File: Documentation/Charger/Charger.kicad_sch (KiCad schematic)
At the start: 14 parts

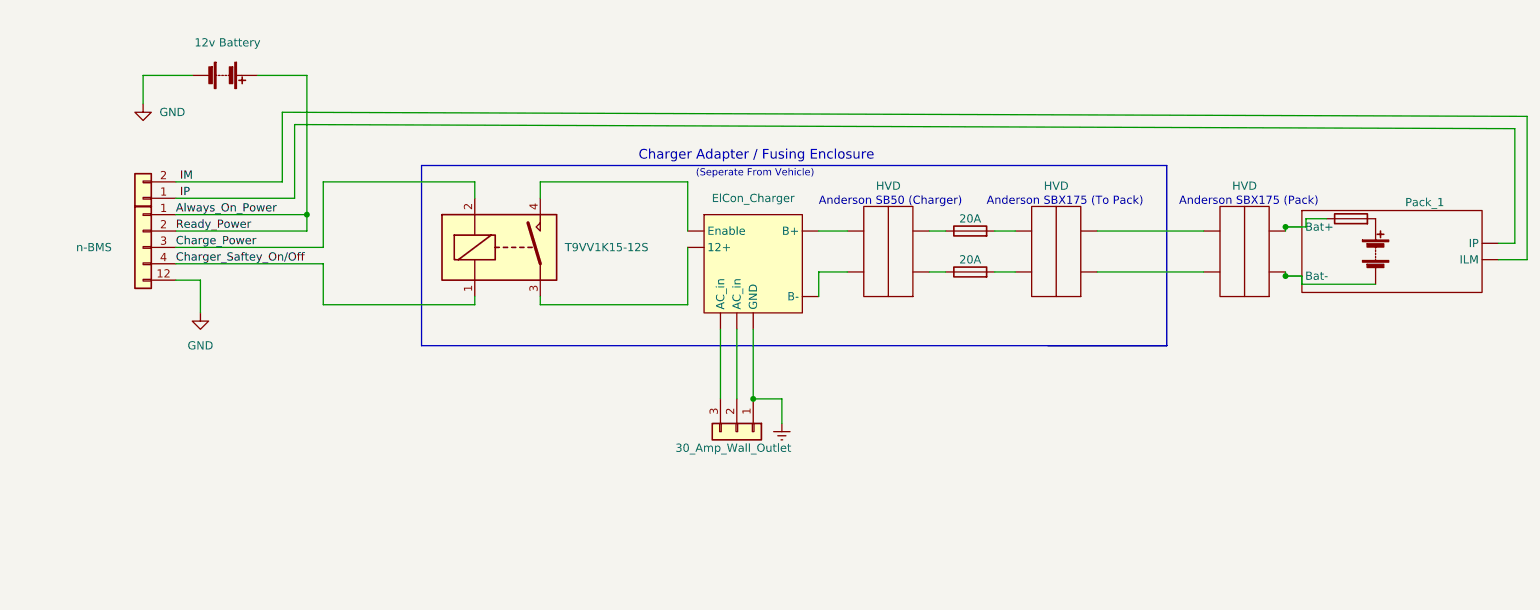
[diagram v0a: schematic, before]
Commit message: end of year DUMP
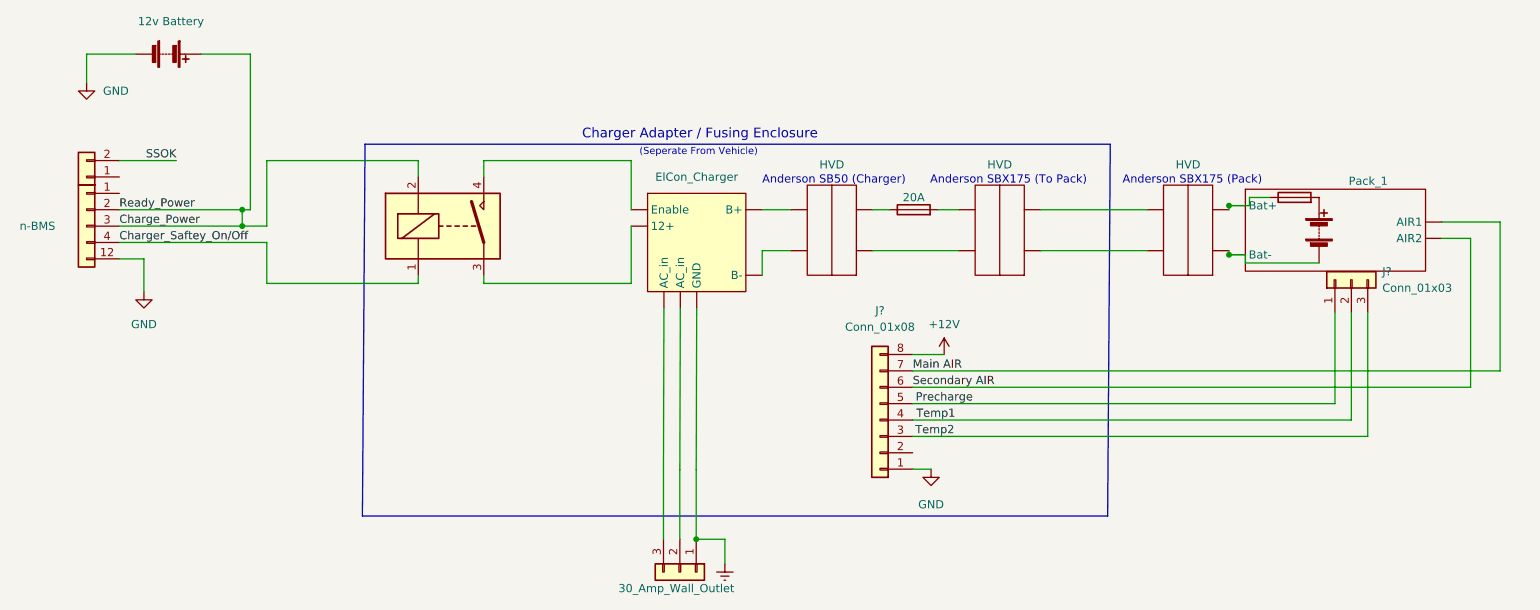
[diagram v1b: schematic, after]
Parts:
- removed F?: 20A, symbol Device:Fuse
- added J?: Conn_01x03, symbol Connector_Generic:Conn_01x03
- added J?: Conn_01x08, symbol Connector_Generic:Conn_01x08
- K?: value T9VV1K15-12S -> (none)
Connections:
- net Charge_Power: now also BT?.1 (+), J?.2 (Pin_2)
- net GND: now also J?.1 (Pin_1)
- net at U?.: now also U?.; no longer U?.
- removed net Always_On_Power: BT?.1 (+), J?.1 (Pin_1), J?.2 (Pin_2)
- net IM renamed SSOK
- net SSOK: no longer U?. (IP)
- net IP: no longer names the net of J?.1 (Pin_1)
- net IP: no longer U?. (IP)
- new net: F?.1, U?., U?. (Bat-)
- new net: BT?.2 (-), U?., U?. (Bat-)
- new net: U?., U?.
- new net: U?., U?. (GND) (x2)
- new net +12V: J?.8 (Pin_8)
- new net Main AIR: J?.7 (Pin_7), U?. (Bat-)
- new net Precharge: J?.1 (Pin_1), J?.5 (Pin_5)
- new net Secondary AIR: J?.6 (Pin_6), U?. (Bat-)
- new net Temp1: J?.2 (Pin_2), J?.4 (Pin_4)
- new net Temp2: J?.3 (Pin_3), J?.3 (Pin_3)
